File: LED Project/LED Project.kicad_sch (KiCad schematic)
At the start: 3 parts, among them J1 Conn_01x02_Pin

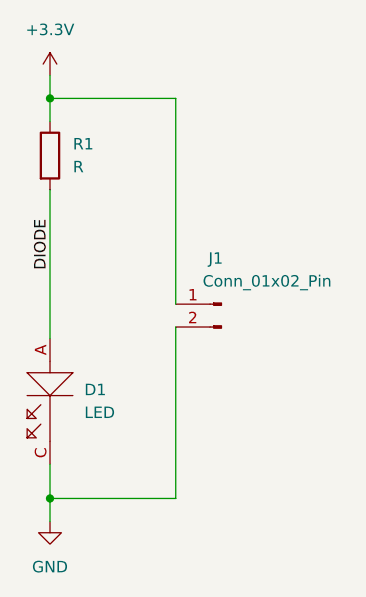
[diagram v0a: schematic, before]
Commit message: ON-OFF-LAMP First Trial
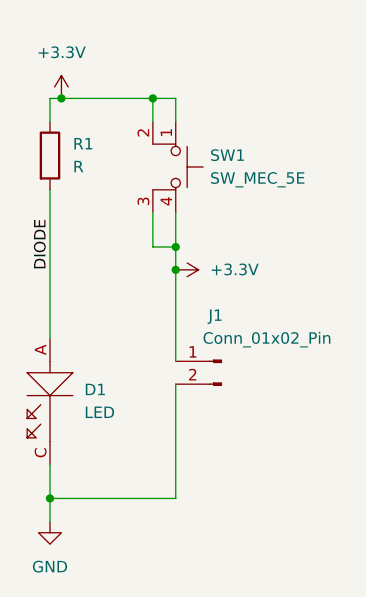
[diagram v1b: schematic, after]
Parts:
- added SW1: SW_MEC_5E, Button_Switch_SMD:SW_SPST_SKQG_WithStem, symbol Switch:SW_MEC_5E
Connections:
- net +3.3V: now also SW1.1, SW1.2, SW1.3 (K), SW1.4 (A)
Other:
- moved on the sheet: J1
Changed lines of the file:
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@@
 (kicad_sch (version 20230121) (generator eeschema)
   (paper "A5")
-  (junction (at 77.47 38.1) (diameter 0) (color 0 0 0 0)
+  (junction (at 91.44 54.61) (diameter 0) (color 0 0 0 0)
   )
   (junction (at 77.47 82.55) (diameter 0) (color 0 0 0 0)
   )
+  (junction (at 78.74 38.1) (diameter 0) (color 0 0 0 0)
+  )
+  (junction (at 88.9 38.1) (diameter 0) (color 0 0 0 0)
+  )
+  (junction (at 91.44 57.15) (diameter 0) (color 0 0 0 0)
+  )
+  (wire (pts (xy 78.74 38.1) (xy 88.9 38.1))
+    (stroke (width 0) (type default))
+  )
+  (wire (pts (xy 91.44 50.8) (xy 91.44 54.61))
+    (stroke (width 0) (type default))
+  )
   (wire (pts (xy 77.47 82.55) (xy 77.47 78.74))
     (stroke (width 0) (type default))
   )
+  (wire (pts (xy 88.9 50.8) (xy 88.9 54.61))
+    (stroke (width 0) (type default))
+  )
   (wire (pts (xy 77.47 48.26) (xy 77.47 64.77))
     (stroke (width 0) (type default))
   )
-  (wire (pts (xy 91.44 38.1) (xy 91.44 60.96))
-    (stroke (width 0) (type default))
-  )
-  (wire (pts (xy 77.47 38.1) (xy 91.44 38.1))
+  (wire (pts (xy 91.44 54.61) (xy 91.44 57.15))
+    (stroke (width 0) (type default))
+  )
+  (wire (pts (xy 77.47 38.1) (xy 78.74 38.1))
     (stroke (width 0) (type default))
   )
@@
     (stroke (width 0) (type default))
   )
-  (wire (pts (xy 77.47 35.56) (xy 77.47 38.1))
+  (wire (pts (xy 88.9 38.1) (xy 91.44 38.1))
     (stroke (width 0) (type default))
   )
@@
     (stroke (width 0) (type default))
   )
-  (wire (pts (xy 91.44 63.5) (xy 91.44 82.55))
-    (stroke (width 0) (type default))
-  )
-  (wire (pts (xy 91.44 82.55) (xy 77.47 82.55))
+  (wire (pts (xy 91.44 38.1) (xy 91.44 40.64))
+    (stroke (width 0) (type default))
+  )
+  (wire (pts (xy 88.9 54.61) (xy 91.44 54.61))
+    (stroke (width 0) (type default))
+  )
+  (wire (pts (xy 91.44 69.85) (xy 91.44 82.55))
+    (stroke (width 0) (type default))
+  )
+  (wire (pts (xy 88.9 38.1) (xy 88.9 40.64))
+    (stroke (width 0) (type default))
+  )
+  (wire (pts (xy 77.47 82.55) (xy 91.44 82.55))
+    (stroke (width 0) (type default))
+  )
+  (wire (pts (xy 91.44 57.15) (xy 91.44 67.31))
     (stroke (width 0) (type default))
   )
@@
     (effects (font (size 1.27 1.27)) (justify left bottom))
   )
-  (symbol (lib_id "Connector:Conn_01x02_Pin") (at 96.52 60.96 0) (mirror y) (unit 1)
+  (symbol (lib_id "Connector:Conn_01x02_Pin") (at 96.52 67.31 0) (mirror y) (unit 1)
     (in_bom yes) (on_board yes) (dnp no)
-    (property "Reference" "J1" (at 95.885 55.88 0)
-      (effects (font (size 1.27 1.27)))
-    )
-    (property "Value" "Conn_01x02_Pin" (at 101.6 58.42 0)
-      (effects (font (size 1.27 1.27)))
-    )
-    (property "Footprint" "Connector_Molex:Molex_KK-254_AE-6410-02A_1x02_P2.54mm_Vertical" (at 96.52 60.96 0)
-      (effects (font (size 1.27 1.27)) hide)
-    )
-    (property "Datasheet" "~" (at 96.52 60.96 0)
+    (property "Reference" "J1" (at 95.885 62.23 0)
+      (effects (font (size 1.27 1.27)))
+    )
+    (property "Value" "Conn_01x02_Pin" (at 101.6 64.77 0)
+      (effects (font (size 1.27 1.27)))
+    )
+    (property "Footprint" "Connector_Molex:Molex_KK-254_AE-6410-02A_1x02_P2.54mm_Vertical" (at 96.52 67.31 0)
+      (effects (font (size 1.27 1.27)) hide)
+    )
+    (property "Datasheet" "~" (at 96.52 67.31 0)
       (effects (font (size 1.27 1.27)) hide)
     )
@@
     )
   )
-  (symbol (lib_id "power:+3.3V") (at 77.47 35.56 0) (unit 1)
-    (in_bom yes) (on_board yes) (dnp no) (fields_autoplaced)
-    (property "Reference" "#PWR01" (at 77.47 39.37 0)
-      (effects (font (size 1.27 1.27)) hide)
-    )
-    (property "Value" "+3.3V" (at 77.47 30.48 0)
-      (effects (font (size 1.27 1.27)))
-    )
-    (property "Footprint" "" (at 77.47 35.56 0)
-      (effects (font (size 1.27 1.27)) hide)
-    )
-    (property "Datasheet" "" (at 77.47 35.56 0)
+  (symbol (lib_id "Switch:SW_MEC_5E") (at 88.9 45.72 270) (unit 1)
+    (in_bom yes) (on_board yes) (dnp no) (fields_autoplaced)
+    (property "Reference" "SW1" (at 95.25 44.45 90)
+      (effects (font (size 1.27 1.27)) (justify left))
+    )
+    (property "Value" "SW_MEC_5E" (at 95.25 46.99 90)
+      (effects (font (size 1.27 1.27)) (justify left))
+    )
+    (property "Footprint" "Button_Switch_SMD:SW_SPST_SKQG_WithStem" (at 96.52 45.72 0)
+      (effects (font (size 1.27 1.27)) hide)
+    )
+    (property "Datasheet" "http://www.apem.com/int/index.php?controller=attachment&id_attachment=1371" (at 96.52 45.72 0)
+      (effects (font (size 1.27 1.27)) hide)
+    )
+    (pin "1")
+    (pin "2")
+    (pin "3")
+    (pin "4")
+    (instances
+      (project "LED Project"
+        (path "/86cec6ac-39e1-4f10-b263-ad2e2393d114"
+          (reference "SW1") (unit 1)
+        )
+      )
+    )
+  )
+  (symbol (lib_id "power:+3.3V") (at 91.44 57.15 270) (unit 1)
+    (in_bom yes) (on_board yes) (dnp no) (fields_autoplaced)
+    (property "Reference" "#PWR03" (at 87.63 57.15 0)
+      (effects (font (size 1.27 1.27)) hide)
+    )
+    (property "Value" "+3.3V" (at 95.25 57.15 90)
+      (effects (font (size 1.27 1.27)) (justify left))
+    )
+    (property "Footprint" "" (at 91.44 57.15 0)
+      (effects (font (size 1.27 1.27)) hide)
+    )
+    (property "Datasheet" "" (at 91.44 57.15 0)
+      (effects (font (size 1.27 1.27)) hide)
+    )
+    (pin "1")
+    (instances
+      (project "LED Project"
+        (path "/86cec6ac-39e1-4f10-b263-ad2e2393d114"
+          (reference "#PWR03") (unit 1)
+        )
+      )
+    )
+  )
+  (symbol (lib_id "Device:R") (at 77.47 44.45 0) (unit 1)
+    (in_bom yes) (on_board yes) (dnp no) (fields_autoplaced)
+    (property "Reference" "R1" (at 80.01 43.18 0)
+      (effects (font (size 1.27 1.27)) (justify left))
+    )
+    (property "Value" "R" (at 80.01 45.72 0)
+      (effects (font (size 1.27 1.27)) (justify left))
+    )
+    (property "Footprint" "Resistor_SMD:R_0805_2012Metric" (at 75.692 44.45 90)
+      (effects (font (size 1.27 1.27)) hide)
+    )
+    (property "Datasheet" "~" (at 77.47 44.45 0)
+      (effects (font (size 1.27 1.27)) hide)
+    )
+    (pin "1")
+    (pin "2")
+    (instances
+      (project "LED Project"
+        (path "/86cec6ac-39e1-4f10-b263-ad2e2393d114"
+          (reference "R1") (unit 1)
+        )
+      )
+    )
+  )
+  (symbol (lib_id "power:+3.3V") (at 78.74 38.1 0) (unit 1)
+    (in_bom yes) (on_board yes) (dnp no) (fields_autoplaced)
+    (property "Reference" "#PWR01" (at 78.74 41.91 0)
+      (effects (font (size 1.27 1.27)) hide)
+    )
+    (property "Value" "+3.3V" (at 78.74 33.02 0)
+      (effects (font (size 1.27 1.27)))
+    )
+    (property "Footprint" "" (at 78.74 38.1 0)
+      (effects (font (size 1.27 1.27)) hide)
+    )
+    (property "Datasheet" "" (at 78.74 38.1 0)
       (effects (font (size 1.27 1.27)) hide)
     )
@@
         )
       )
-    )
-  )
-  (symbol (lib_id "Device:R") (at 77.47 44.45 0) (unit 1)
-    (in_bom yes) (on_board yes) (dnp no) (fields_autoplaced)
-    (property "Reference" "R1" (at 80.01 43.18 0)
-      (effects (font (size 1.27 1.27)) (justify left))
-    )
-    (property "Value" "R" (at 80.01 45.72 0)
-      (effects (font (size 1.27 1.27)) (justify left))
-    )
-    (property "Footprint" "Resistor_SMD:R_0805_2012Metric" (at 75.692 44.45 90)
-      (effects (font (size 1.27 1.27)) hide)
-    )
-    (property "Datasheet" "~" (at 77.47 44.45 0)
-      (effects (font (size 1.27 1.27)) hide)
-    )
-    (pin "1")
-    (pin "2")
-    (instances
-      (project "LED Project"
-        (path "/86cec6ac-39e1-4f10-b263-ad2e2393d114"
-          (reference "R1") (unit 1)
-        )
-      )
